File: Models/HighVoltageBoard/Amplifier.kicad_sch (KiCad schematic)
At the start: 13 parts, among them J4 Conn_01x03_Socket, J8 Conn_Coaxial, Q1 Q_NJFET_DSG, Q5 Q_NJFET_DSG, U1 PA95

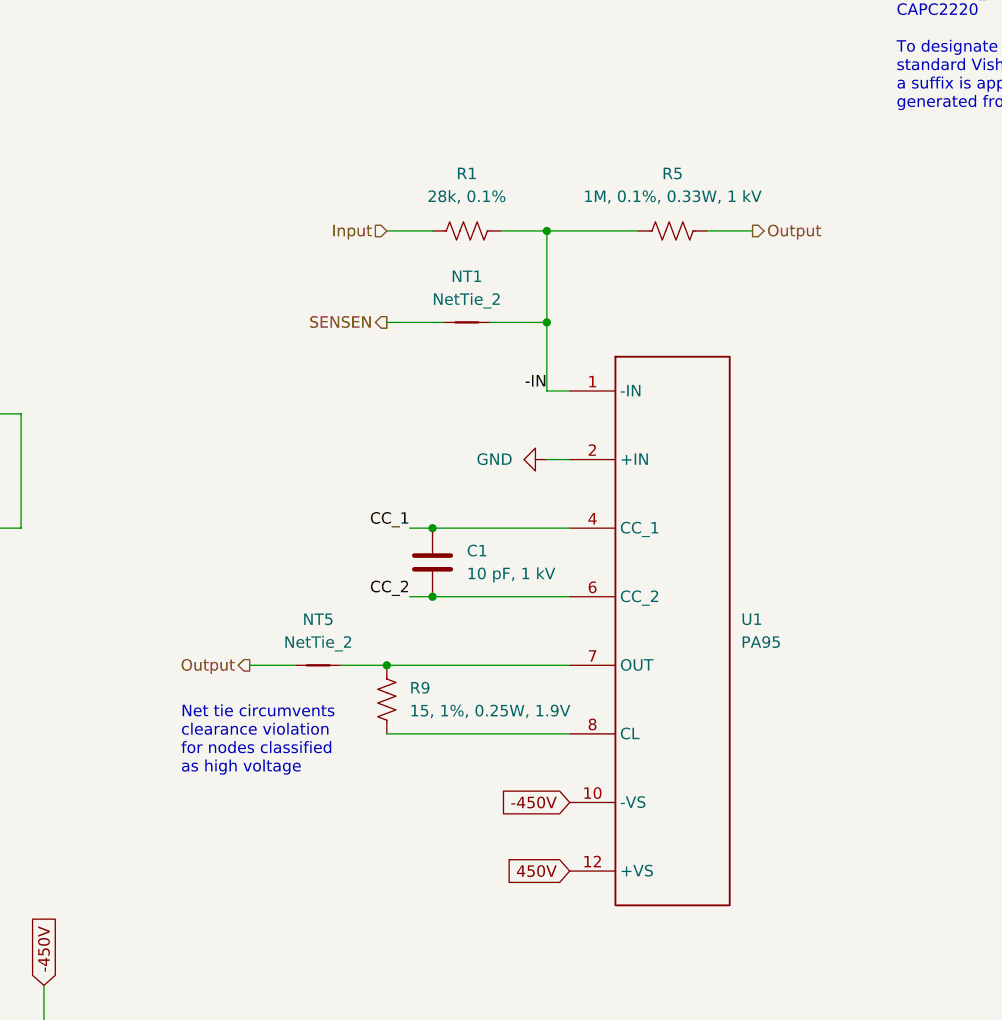
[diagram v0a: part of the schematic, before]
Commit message: Save progress
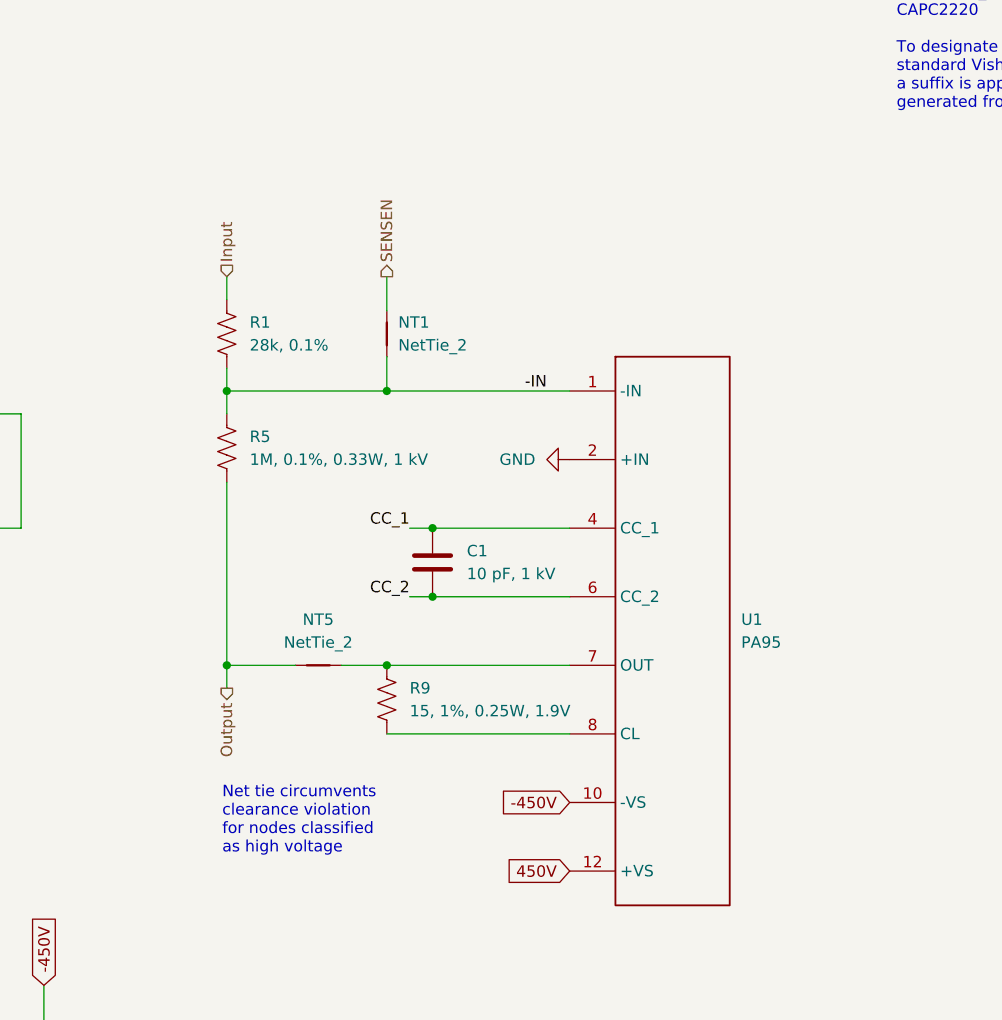
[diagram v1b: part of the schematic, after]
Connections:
- net -IN: now also NT1.1; no longer NT1.2
- net SENSEN: now also NT1.2; no longer NT1.1
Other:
- moved on the sheet: NT1, R1, R5
